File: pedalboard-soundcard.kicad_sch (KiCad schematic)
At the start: 21 parts, among them J1 RPi_GPIO, U1 AT24CS01-STUM, U2 ncp163, U3 ncp163, U5 ncp163

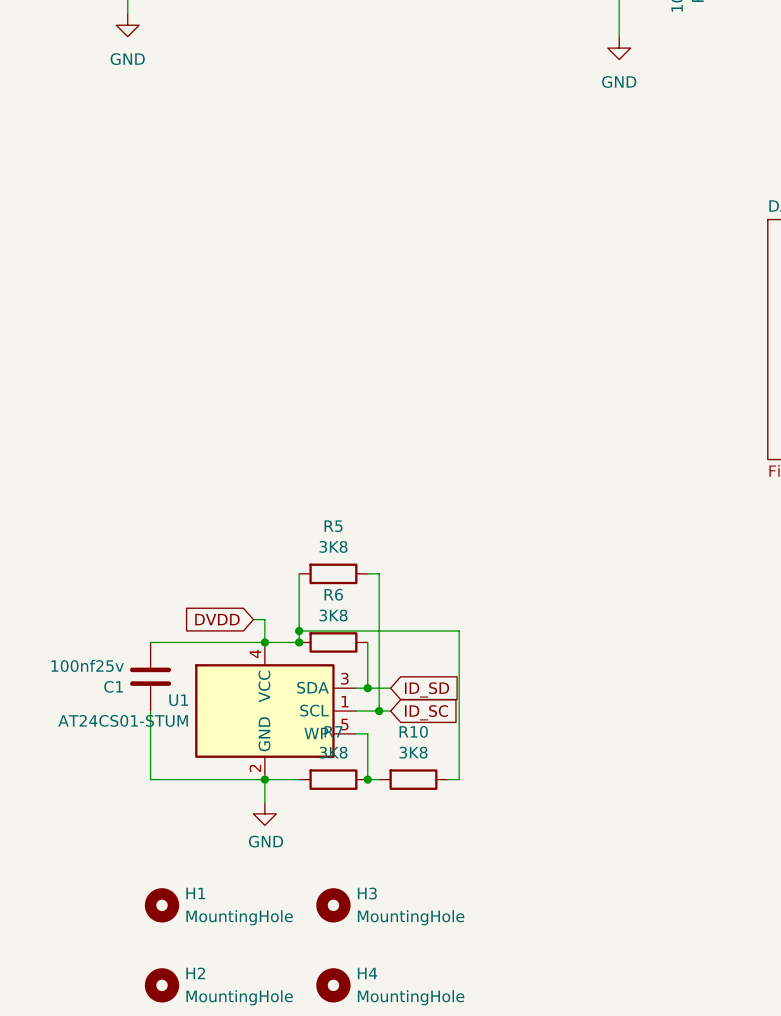
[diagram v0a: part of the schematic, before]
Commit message: Distribute parts on PCB
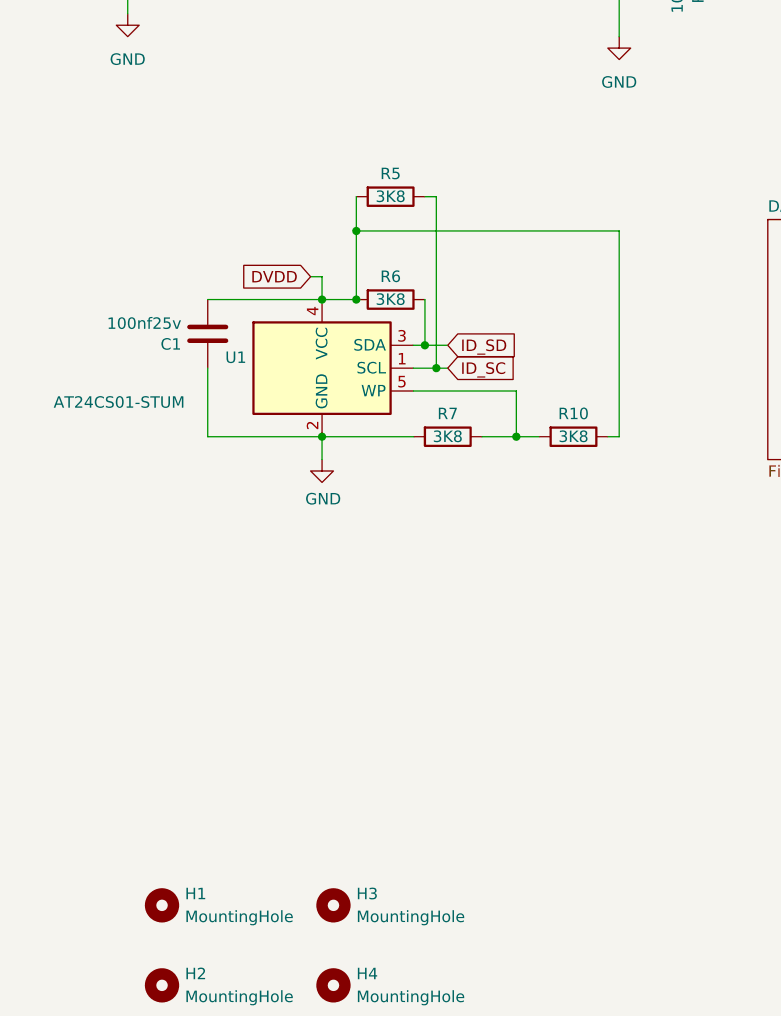
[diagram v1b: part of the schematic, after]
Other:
- moved on the sheet: C1, R10, R5, R6, R7, U1

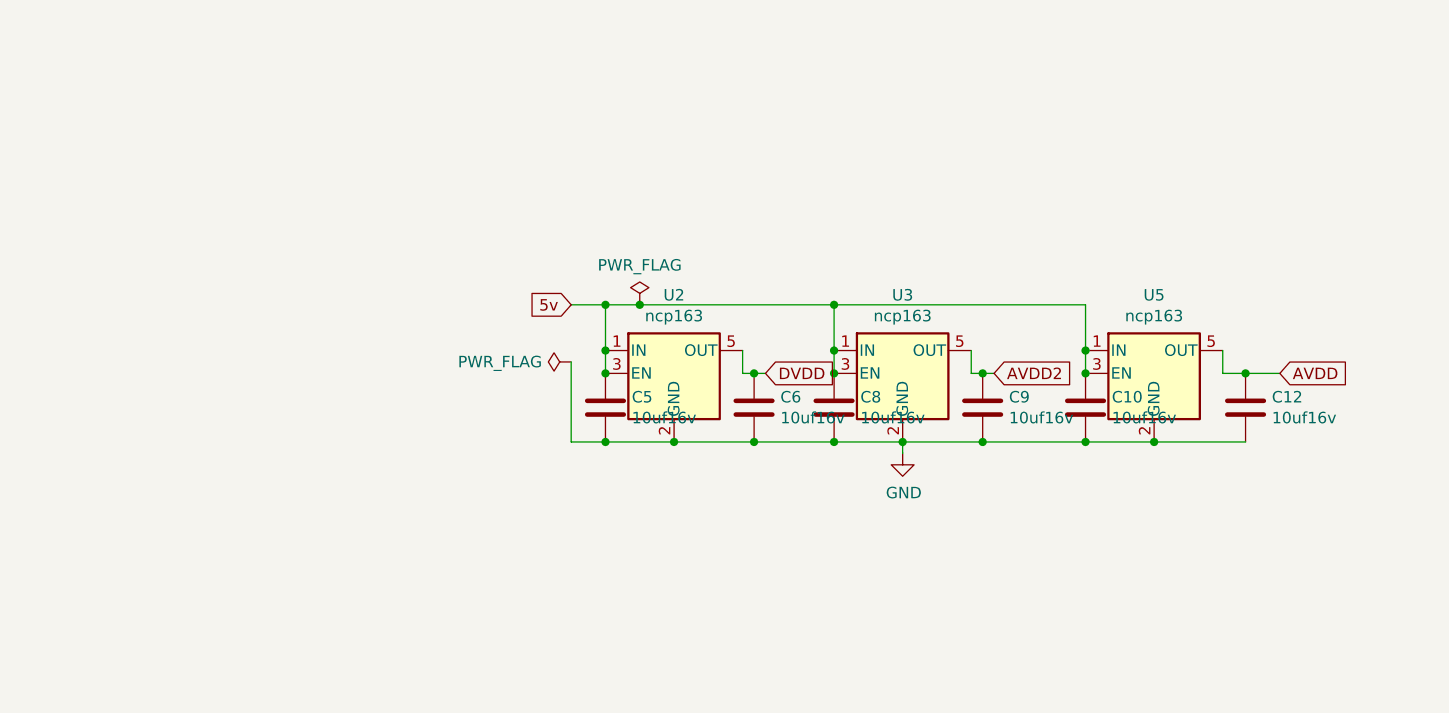
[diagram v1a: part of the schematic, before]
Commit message: Cleanup placement
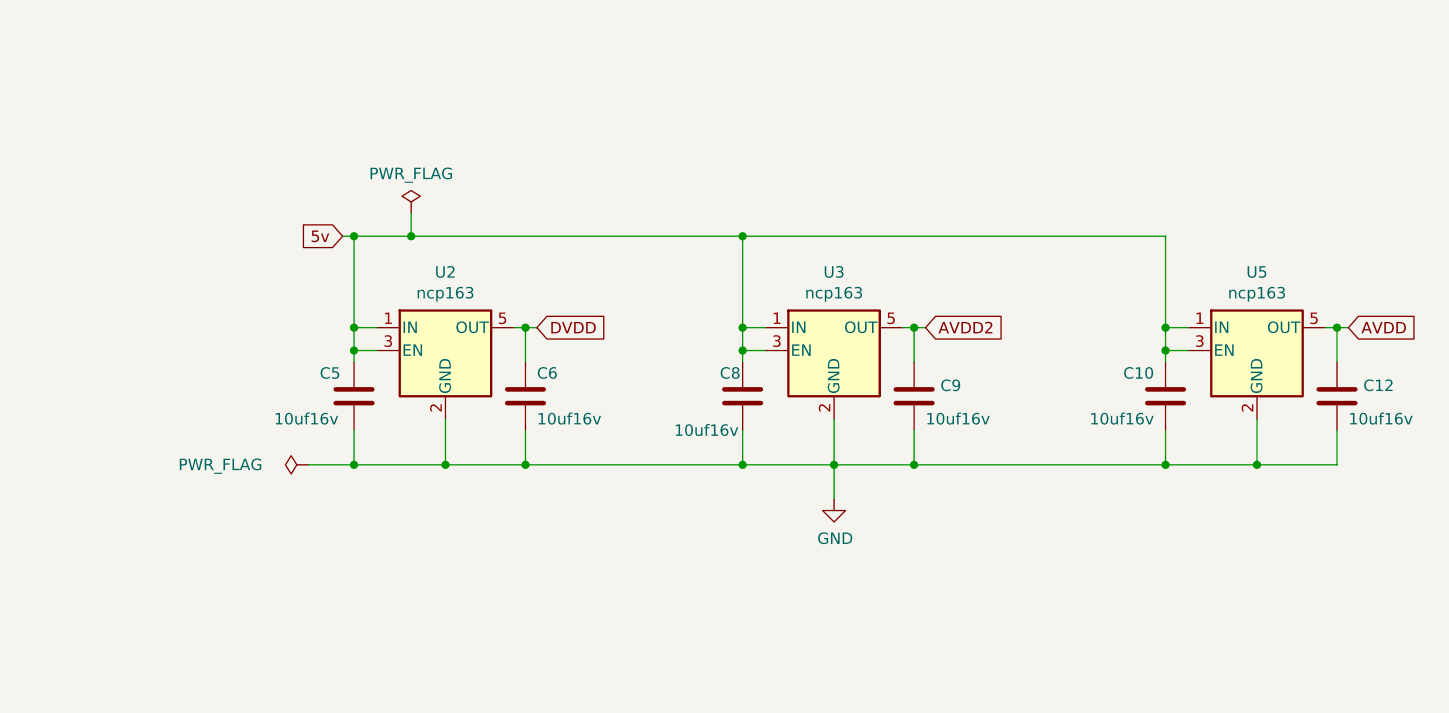
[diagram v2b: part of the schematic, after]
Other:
- moved on the sheet: C10, C12, C5, C6, C8, C9, U2, U3, U5
